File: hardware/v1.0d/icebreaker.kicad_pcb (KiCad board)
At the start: 4 copper layers, 73 x 37 mm, 191 parts, among them J1 Jumper, J10 Jumper, J11 Jumper, J12 Jumper, J13 Jumper, J14 Jumper, J15 Jumper, J16 Jumper, J17 Jumper, J18 Jumper, J19 Jumper, J2 Jumper, J20 Flash, J21 PMOD, J22 PMOD, J23 PMOD, J24 PMOD, J25 RGB Led, J26 5V AUX, J27 5V AUX, J28 CRESET, J29 Jumper, J3 Jumper, J30 Jumper, J31 RGB Led, J32 WS2812, J33 RGB Led, J34 SADD, J4 Jumper, J5 Jumper, J6 Jumper, J7 Jumper, J8 Jumper, J9 Jumper, P1 pkl_USB_OTG, P2 UP, P3 UP, P4 UP, P5 UP, P6 RAM_CS, Q1 BSS138, SW1 TACT, SW2 TACT, SW3 TACT, SW4 TACT, U1 93C46B-SOT-23-6, U2 3.3V, U3 1V2, U4 FT2232H, U5 W25Q, U6 ICE5LP4K-SG48, U7 12MHz

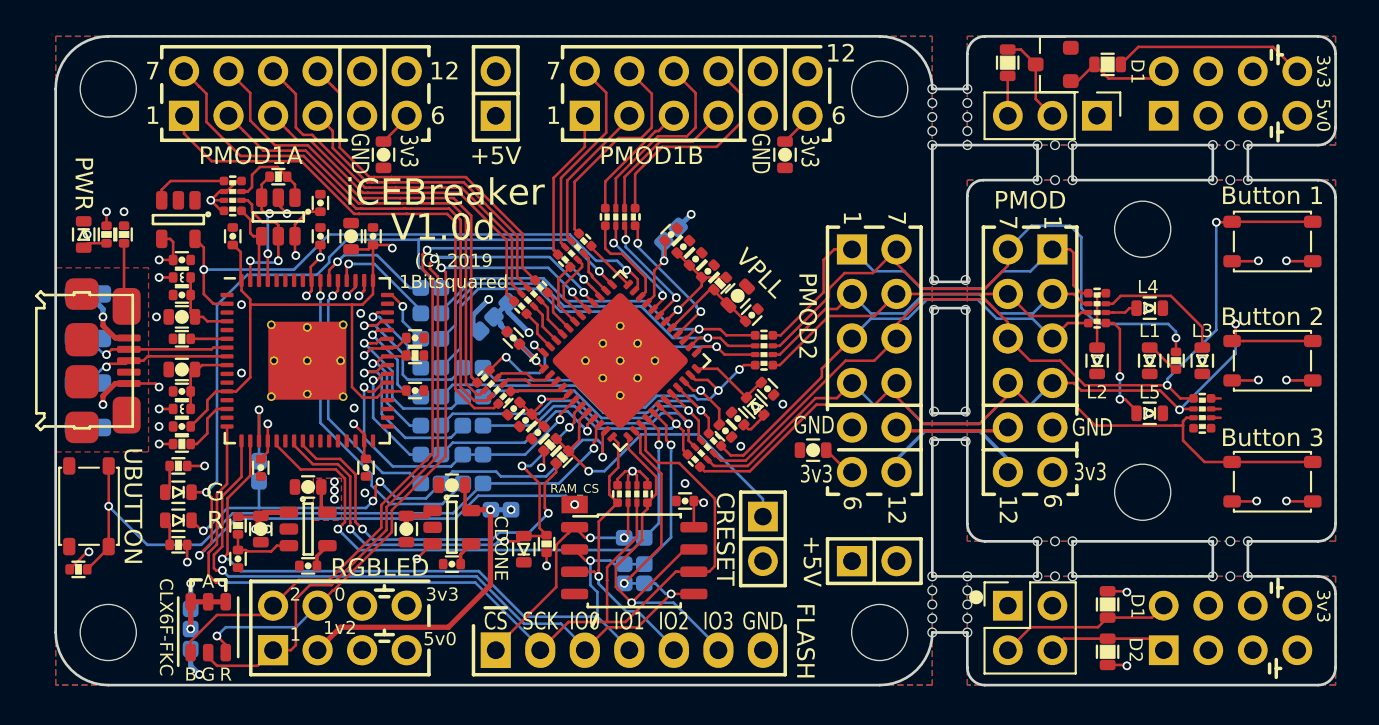
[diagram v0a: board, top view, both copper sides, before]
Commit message: A bunch of DRC fixes and improvements.
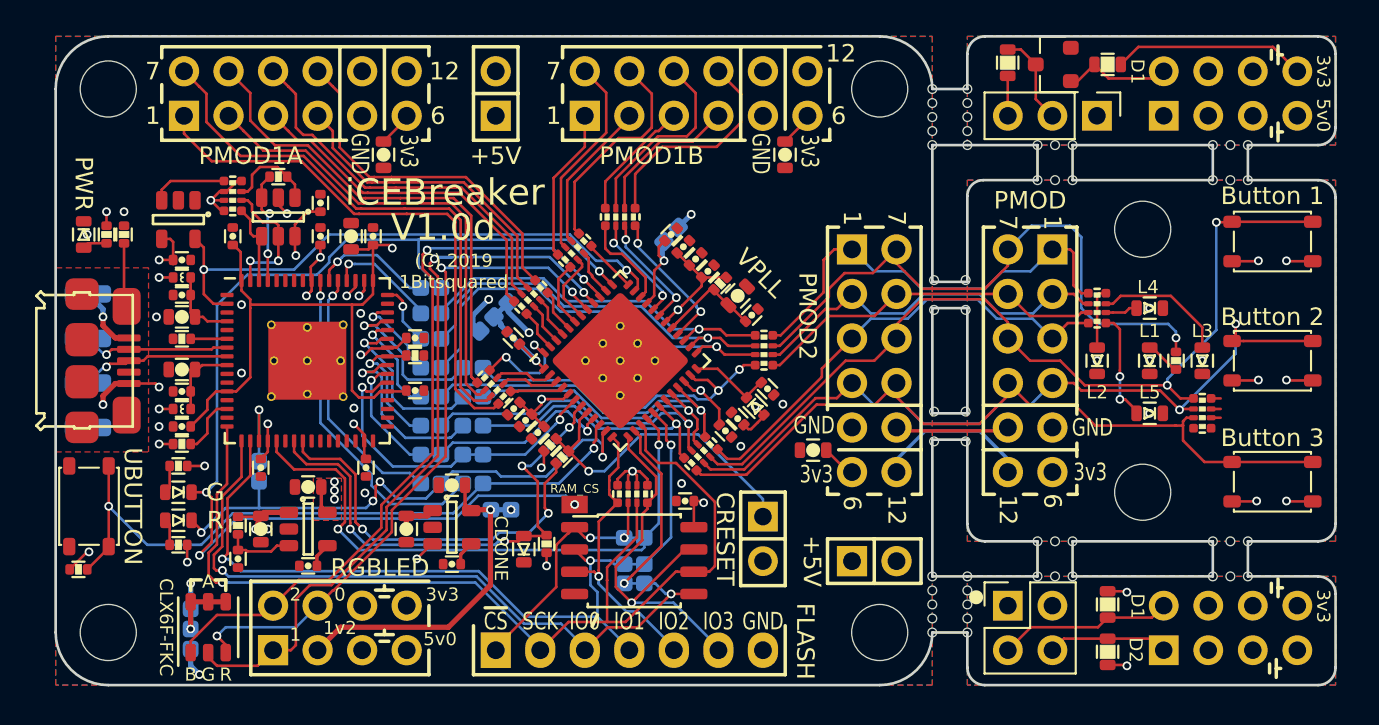
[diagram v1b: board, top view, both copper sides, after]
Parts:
- moved R22 0.28 mm to (66.8, 52.8)
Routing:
- net /iCE_SS_B: track 33.7 -> 34.2 mm
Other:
- net class Default: clearance 0.149 -> 0.15
- rule trace_clearance: 0.149 -> 0.15
- rule trace_min: 0.149 -> 0.15
